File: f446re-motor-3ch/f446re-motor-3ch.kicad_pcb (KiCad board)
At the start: 2 copper layers, 90 x 80 mm, 54 parts, among them J1 電源コネクタ, J2 デバッグ用端子, J3 CANコネクタ, J4 CH1 モータ, J5 CH1 エンコーダ, J6 CH2 モータ, J7 CH2 エンコーダ, J8 CH3 モータ, J9 CH3 エンコーダ, SW1 リセットスイッチ, U1 STM32F446RETx, U2 AZ1117CH-3_3TRG1, U3 MCP2562-E-SN, Y1 Crystal_GND24

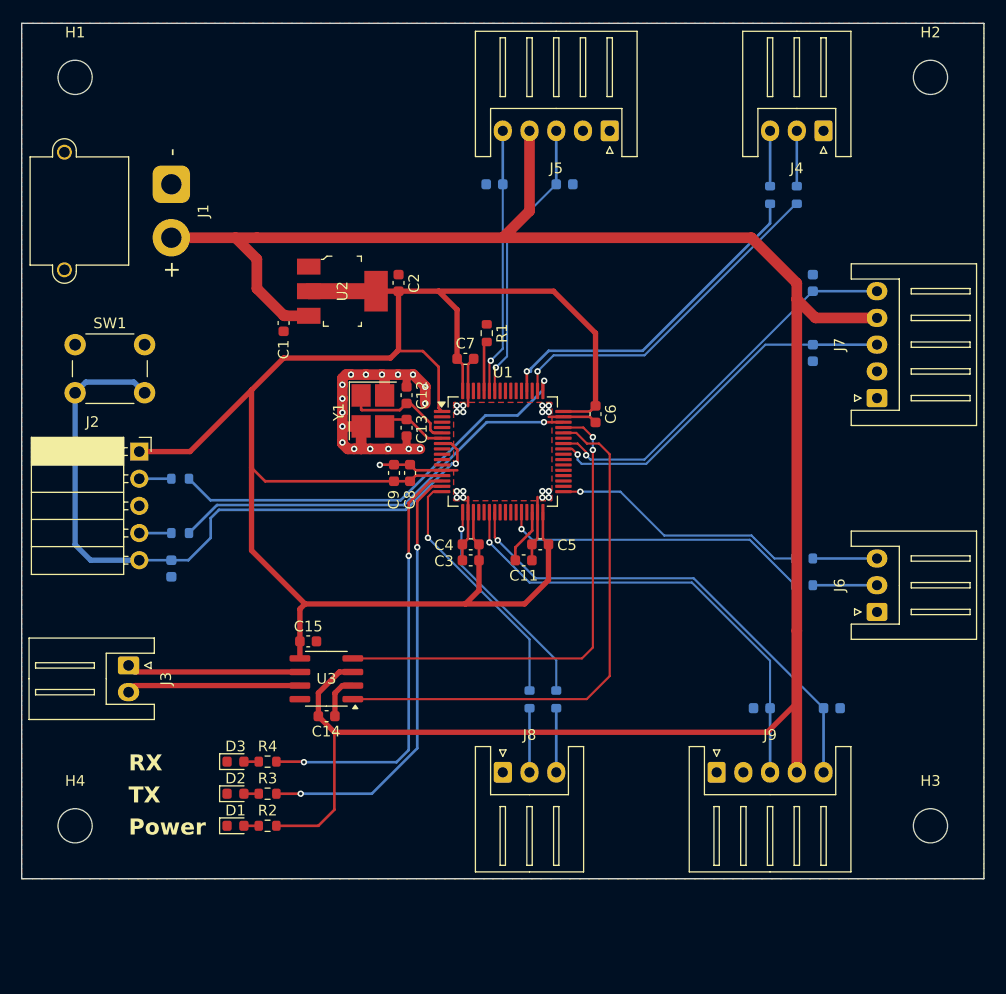
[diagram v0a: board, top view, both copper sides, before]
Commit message: 2025/02/03/12:25
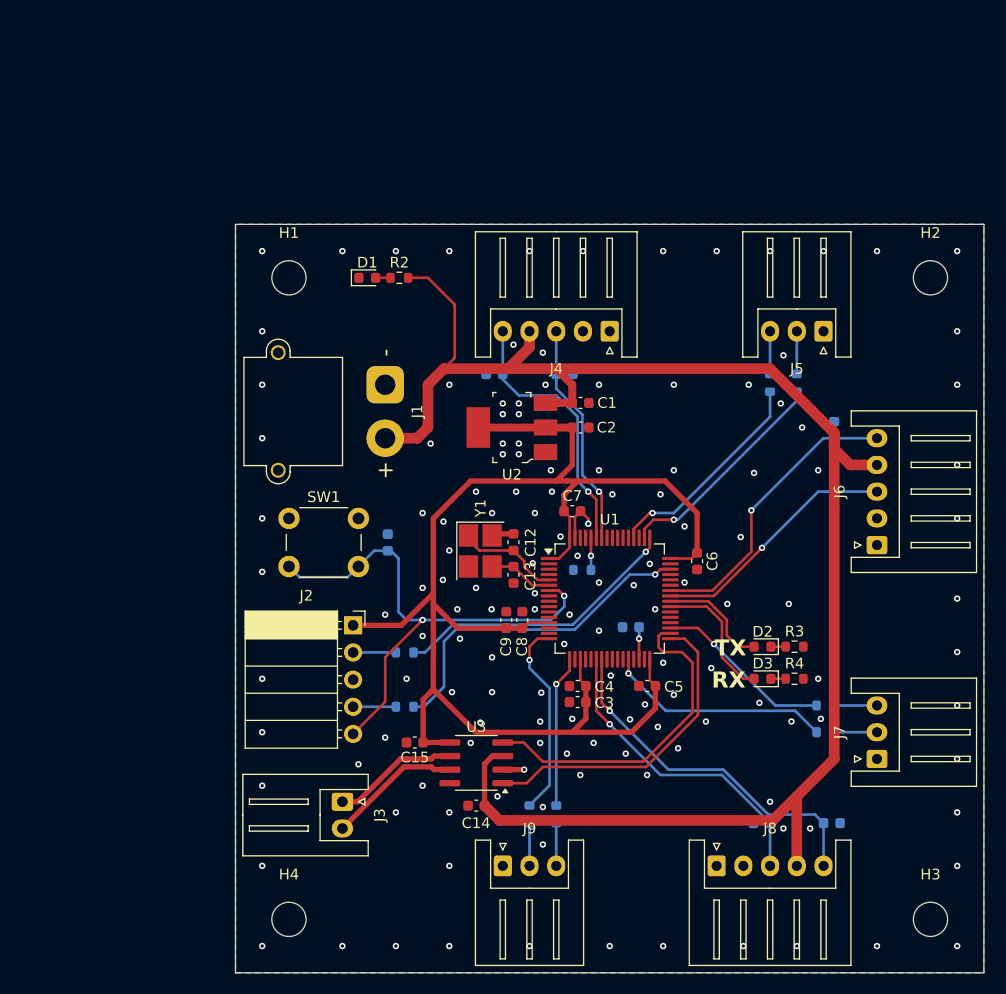
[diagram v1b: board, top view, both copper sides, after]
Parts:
- C11, R1: moved to B.Cu
- C12, C13: value C -> 15pF
- moved D1 52.7 mm to (143.3, 72.0)
- moved R2 52.7 mm to (146.3, 72.0)
- moved D2 51.2 mm to (180.3, 106.5), turned to 180 degrees
- moved R3 51.2 mm to (183.3, 106.5)
- moved D3 49.9 mm to (180.3, 109.5), turned to 180 degrees
- moved R4 49.9 mm to (183.3, 109.5)
- moved C1 28.8 mm to (163.3, 83.7), turned to 0 degrees
- moved H1 27.4 mm to (136.0, 72.0)
- moved J1 27.4 mm to (145.0, 82.0)
- moved R7 26.6 mm to (146.8, 107.0)
- moved R8 26.6 mm to (146.8, 112.1)
- moved J2 25.8 mm to (142.0, 104.5)
- moved SW1 25.8 mm to (136.0, 94.5)
- moved R1 23.9 mm to (163.4, 99.3), turned to 0 degrees
- moved J3 23.7 mm to (141.0, 121.0)
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- renumbered J5 to J4, J4 to J5, J7 to J6, J6 to J7, J9 to J8, J8 to J9
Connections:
- net CAN_H renamed CAN+
- net CAN_L renamed CAN-
- D2 pad 1: GND -> Net-(D2-K)
- D2 pad 2: Net-(D2-A) -> CAN_TX_LED
- D3 pad 1: GND -> Net-(D3-K)
- D3 pad 2: Net-(D3-A) -> CAN_RX_LED
- R3 pad 1: CAN_TX_LED -> GND
- R3 pad 2: Net-(D2-A) -> Net-(D2-K)
- R4 pad 1: CAN_RX_LED -> GND
- R4 pad 2: Net-(D3-A) -> Net-(D3-K)
- U1 pad 14: CAN_RX_LED -> unconnected-(U1-PA0-Pad14)
- U1 pad 15: CAN_TX_LED -> unconnected-(U1-PA1-Pad15)
- U1 pad 33: CH2_MOTOR_DIR -> CAN_RX
- U1 pad 34: unconnected-(U1-PB13-Pad34) -> CAN_TX
- U1 pad 35: unconnected-(U1-PB14-Pad35) -> CH2_MOTOR_DIR
- U1 pad 39: unconnected-(U1-PC8-Pad39) -> CAN_RX_LED
- U1 pad 40: unconnected-(U1-PC9-Pad40) -> CAN_TX_LED
- U1 pad 44: CAN_RX -> unconnected-(U1-PA11-Pad44)
- U1 pad 45: CAN_TX -> unconnected-(U1-PA12-Pad45)
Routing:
- net GND: track 65.2 -> 8.25 mm, vias 34 -> 144
- net +5V: track 209.5 -> 156.7 mm
- net +3.3V: track 176.7 -> 137.9 mm
- net CAN_TX_LED: track 40.9 -> 10.4 mm, vias 2 -> 0
- net CAN_RX_LED: track 39.9 -> 12.5 mm, vias 2 -> 0
- net CAN_RX: track 50.8 -> 29.9 mm
- net NRST: track 65.6 -> 49.3 mm, vias 1 -> 2
- net CH3_ENC_A: track 44.1 -> 29.4 mm
- net CAN_TX: track 45.7 -> 31.1 mm, vias 2 -> 0
- net SWCLK: track 40.1 -> 27.1 mm
- net CH3_ENC_B: track 45.7 -> 33.5 mm
- net CH1_MOTOR_DIR: track 32.3 -> 20.3 mm
- net CH1_MOTOR_PWM: track 32.6 -> 20.9 mm
- net CH2_ENC_A: track 34.8 -> 23.4 mm
- net CH2_ENC_B: track 36.6 -> 27.5 mm
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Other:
- board size 90 x 80 mm -> 70 x 70 mm
- board text removed: "Power"
